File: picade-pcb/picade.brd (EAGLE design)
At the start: 76 x 50 mm, 60 parts, among them P1JOY 2.54MM-5P-SCREW-TERMINALLOCK, P2JOY 2.54MM-5P-SCREW-TERMINALLOCK

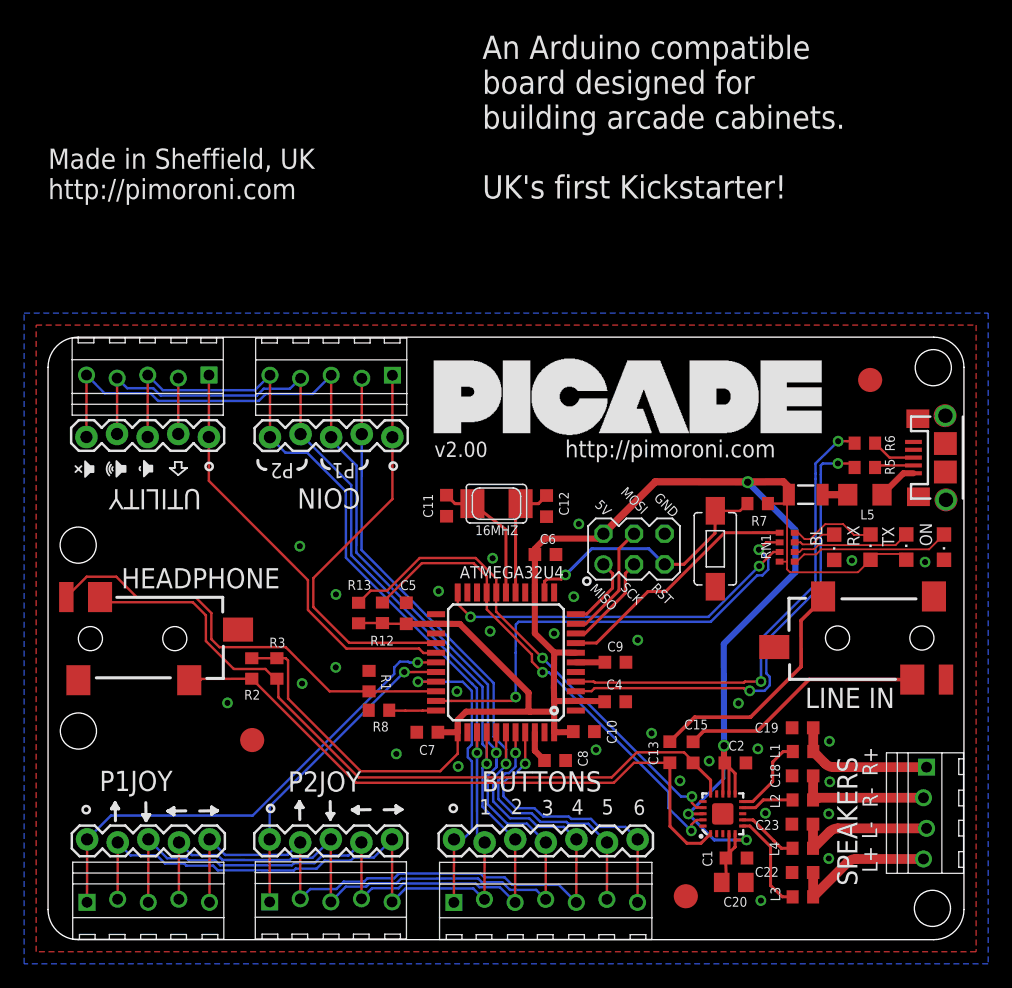
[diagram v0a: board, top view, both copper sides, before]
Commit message: Picade retail board V2.01
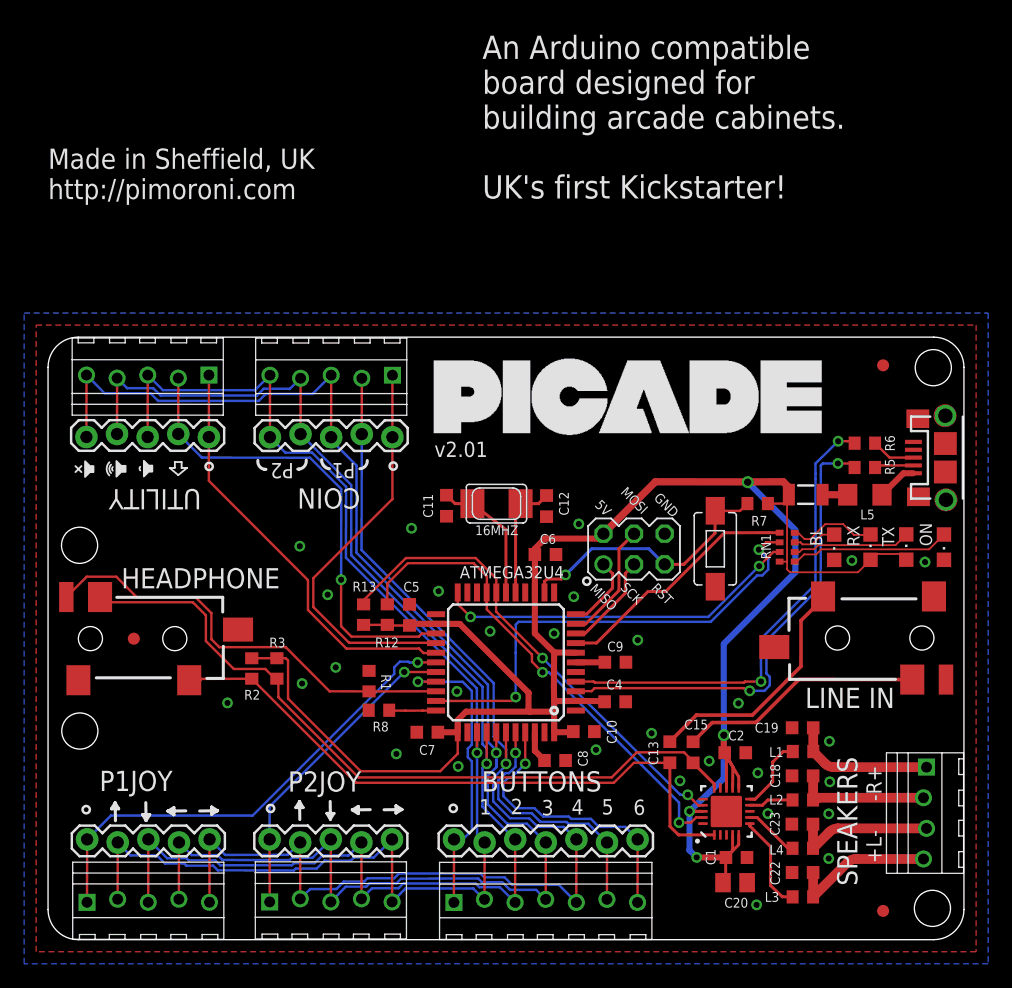
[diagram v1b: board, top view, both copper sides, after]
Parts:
- U$1, U$2, U$3: value FIDUCIAL2MM -> FIDUCIAL1MM; device pimoroni:FIDUCIAL-2MM -> pimoroni:FIDUCIAL-1MM
- U$5: device pimoroni:QFN20 -> pimoroni:TPA2016
- moved U$1 47.0 mm to (69.3, 47.7)
- moved U$2 44.1 mm to (69.3, 2.39)
- moved U$3 12.9 mm to (7.11, 25.0)
- moved C2 0.85 mm to (57.0, 15.5)
- moved R13 0.43 mm to (26.2, 27.0)
- moved R12 0.43 mm to (28.1, 27.0)
- moved C5 0.30 mm to (30.0, 27.0)
- moved C20 0.11 mm to (57.0, 4.73)
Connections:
- net MODESHIFT: now also ATMEGA32U4.25
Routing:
- net MODESHIFT: track 4.63 -> 39.8 mm, vias 0 -> 1
- net OUTR-: track 4.41 -> 3.73 mm
- net OUTR+: track 6.83 -> 6.15 mm
- net 5V: track 180.1 -> 180.7 mm
- net SCL: track 40.6 -> 40.0 mm
- net OUTL-: track 5.12 -> 4.60 mm
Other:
- board text added: "+L-"
- board text added: "-R+"
- board text added: "v2.01"
- board text removed: "L+"
- board text removed: "L-"
- board text removed: "R+"
- board text removed: "R-"
- board text removed: "http://pimoroni.com"
